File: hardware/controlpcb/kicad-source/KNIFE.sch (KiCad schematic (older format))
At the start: 13 parts, among them P4 WR-TBL_691313710002, U15 74xx08, U16 IFX007T

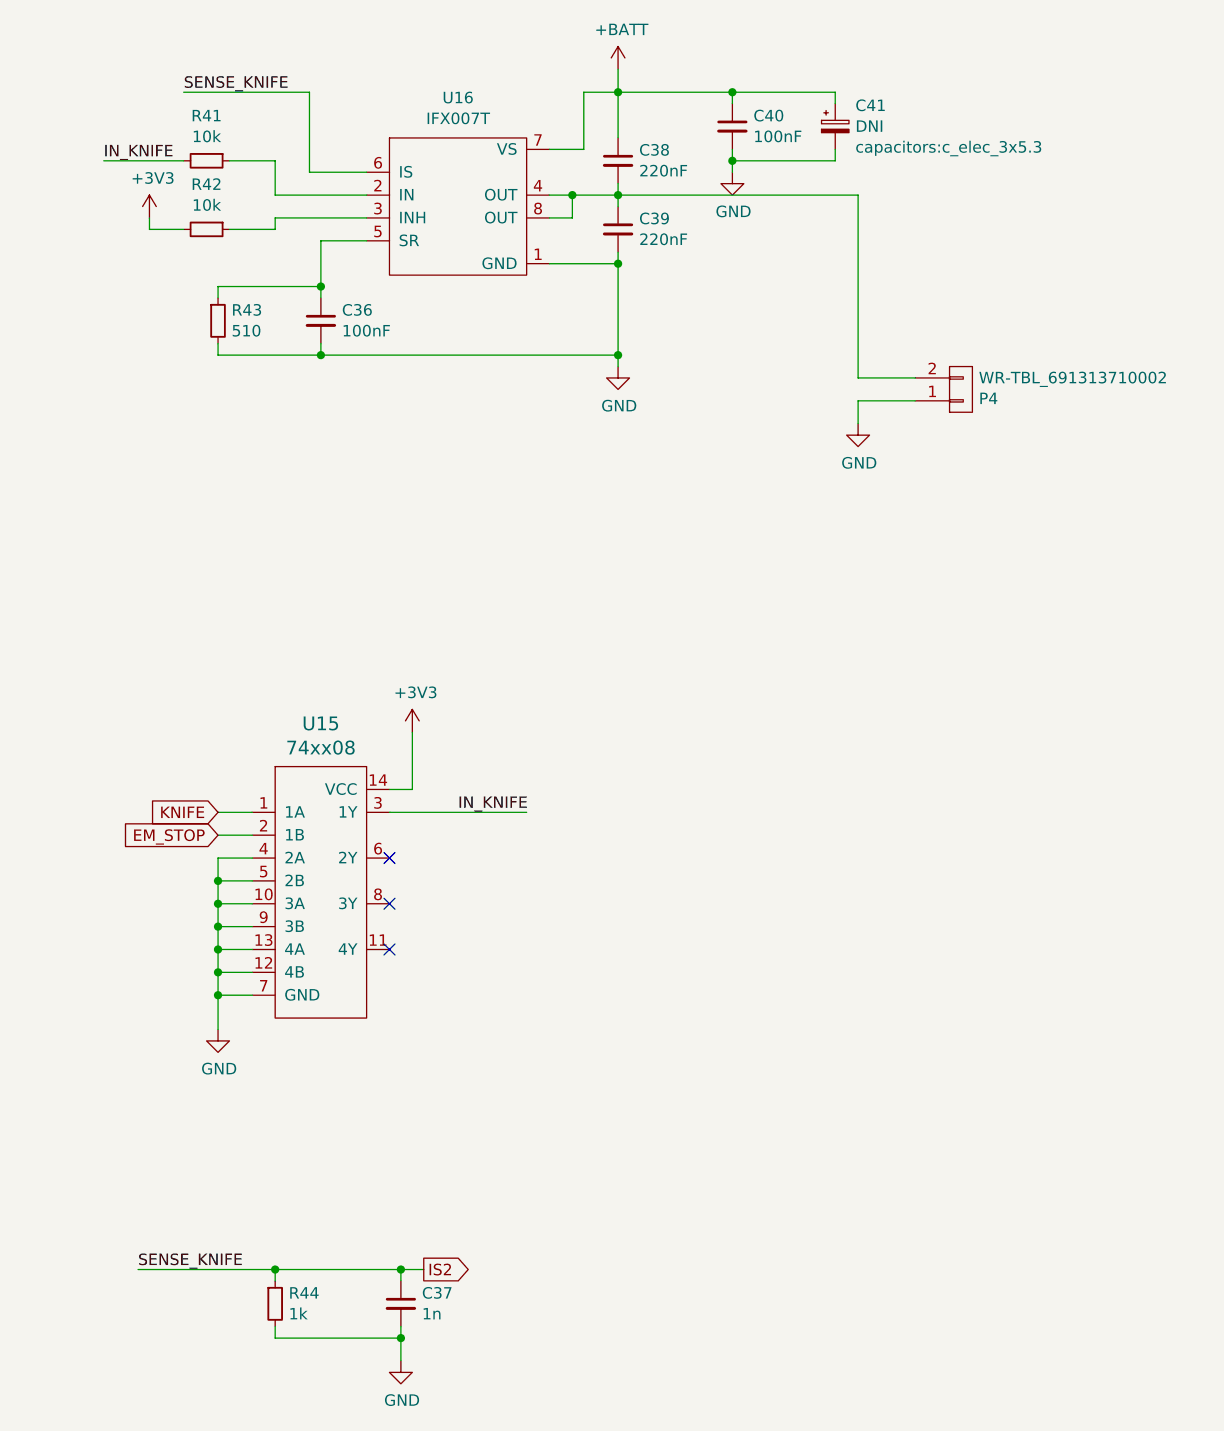
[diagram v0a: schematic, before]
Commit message: added kicad source
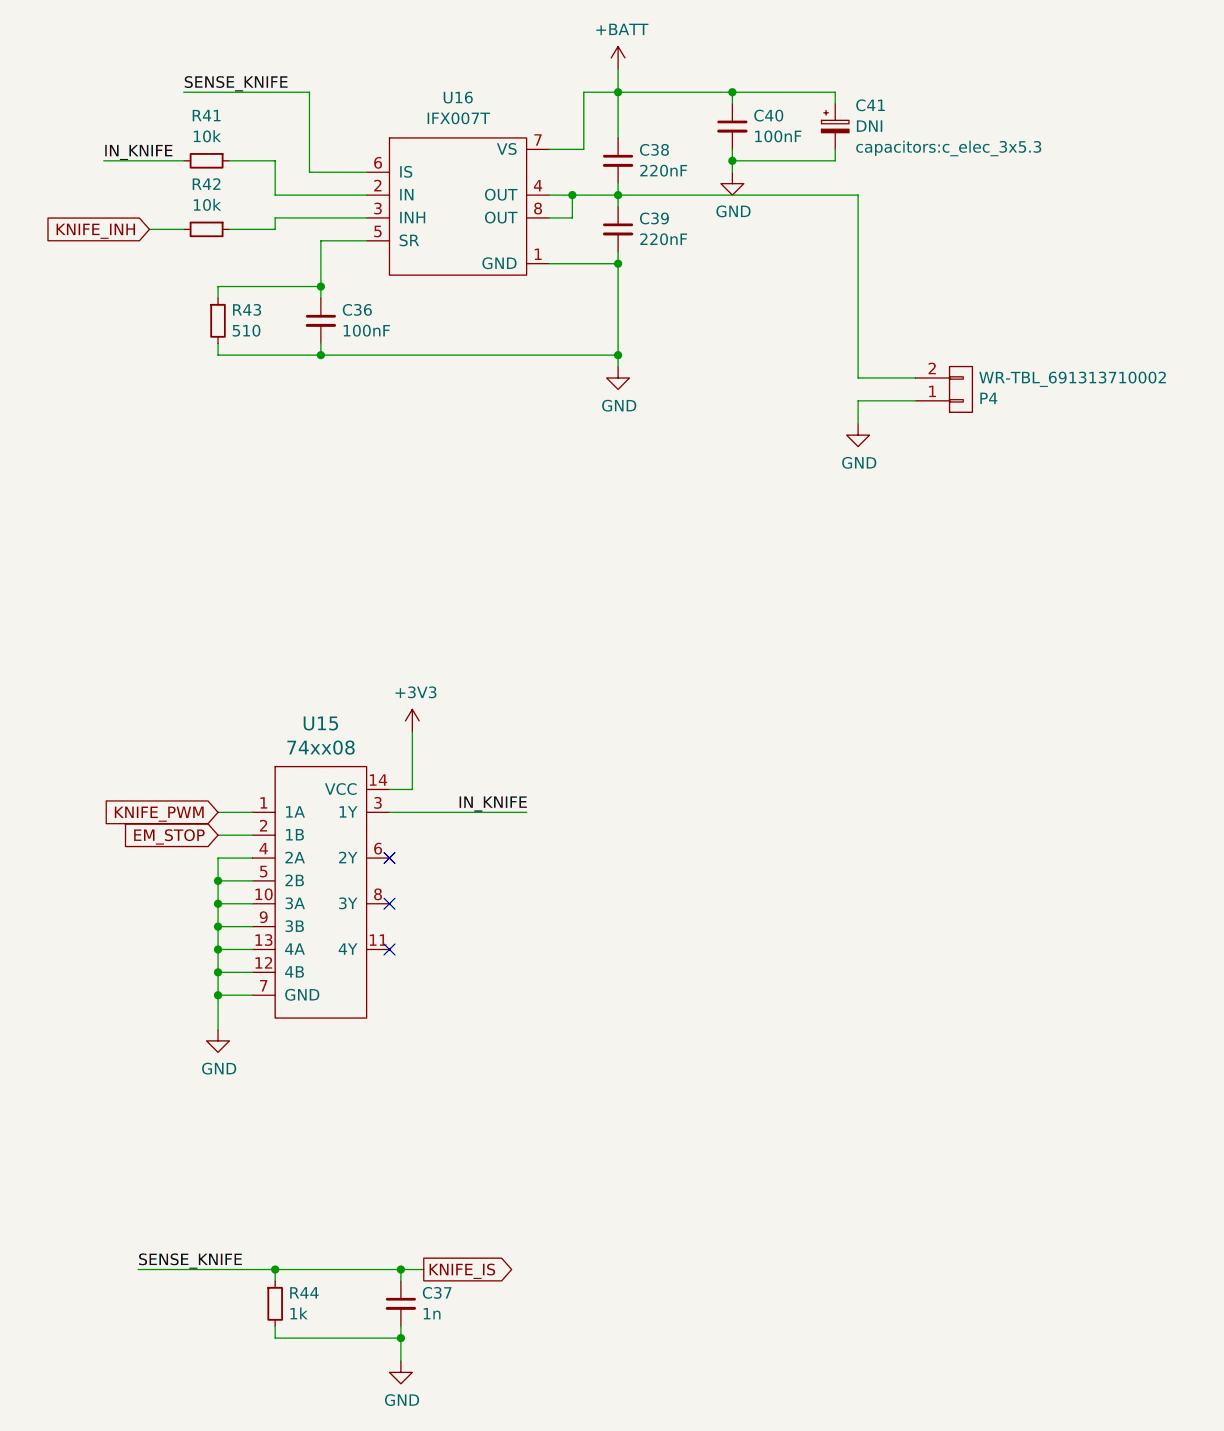
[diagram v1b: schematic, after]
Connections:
- net +3V3: no longer R42.2
- net IS2 renamed KNIFE_IS
- net KNIFE renamed KNIFE_PWM
- new net KNIFE_INH: R42.2
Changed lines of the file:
@@
 IN_KNIFE
-$Comp
-L power-supply:+3V3 #PWR074
-U 1 1 5ECFE999
-P 1900 2000
-F 0 "#PWR074" H 1900 1850 50  0001 C CNN
-F 1 "+3V3" H 1915 2173 50  0000 C CNN
-F 2 "" H 1900 2000 50  0000 C CNN
-F 3 "" H 1900 2000 50  0000 C CNN
-	1    1900 2000
-	1    0    0    -1
-$EndComp
-Wire Wire Line
-	1900 2050 1900 2000
 $Comp
 L IC_logic:74xx08 U15
@@
 EM_STOP
 Text GLabel 2200 4600 0    50   Input ~ 0
-KNIFE
+KNIFE_PWM
 Wire Wire Line
 	2200 4600 2350 4600
@@
 IN_KNIFE
 Text GLabel 3100 6600 2    50   Output ~ 0
-IS2
+KNIFE_IS
 $Comp
 L devices:R_0603 R?
@@
 	1    0    0    1
 $EndComp
+Text GLabel 1900 2050 0    50   Input ~ 0
+KNIFE_INH
 $EndSCHEMATC
